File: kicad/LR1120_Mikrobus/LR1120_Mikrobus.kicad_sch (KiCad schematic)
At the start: 8 parts, among them IC1 BGA524N6E6327XTSA1, IC2 SKY13588-460LF, IC3 M24128-BFMH6TG, U1 LR1120, U4 LIS2DE12

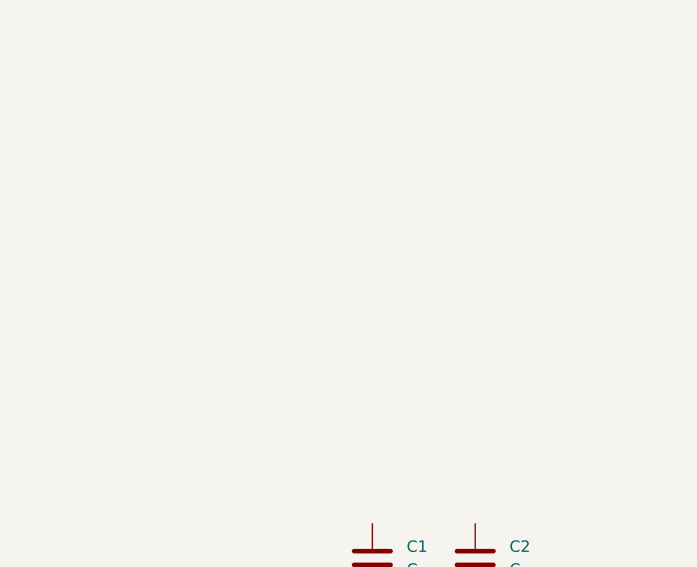
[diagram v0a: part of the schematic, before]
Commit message: Small corrections from last commit
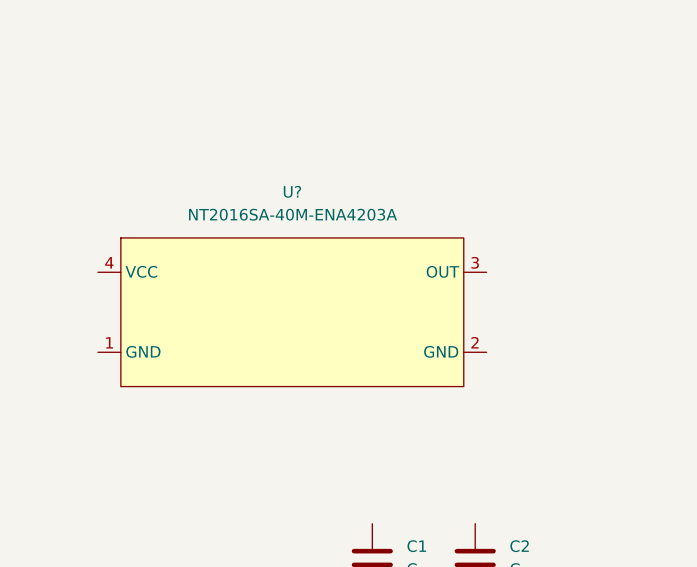
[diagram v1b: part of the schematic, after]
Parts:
- added U?: NT2016SA-40M-ENA4203A, symbol TCXO:NT2016SA-40M-ENA4203A
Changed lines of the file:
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@@
     (pin "9")
+  )
+  (symbol (lib_id "TCXO:NT2016SA-40M-ENA4203A") (at 57.15 66.04 0) (unit 1)
+    (in_bom yes) (on_board yes) (fields_autoplaced)
+    (property "Reference" "U?" (id 0) (at 58.42 53.34 0))
+    (property "Value" "NT2016SA-40M-ENA4203A" (id 1) (at 58.42 55.88 0))
+    (property "Footprint" "" (id 2) (at 57.15 66.04 0)
+      (effects (font (size 1.27 1.27)) hide)
+    )
+    (property "Datasheet" "" (id 3) (at 57.15 66.04 0)
+      (effects (font (size 1.27 1.27)) hide)
+    )
+    (pin "1")
+    (pin "2")
+    (pin "3")
+    (pin "4")
   )
   (symbol (lib_id "M24128-BFMH6TG:M24128-BFMH6TG") (at 233.68 85.09 0) (unit 1)
@@
       (reference "U4") (unit 1) (value "LIS2DE12") (footprint "Package_LGA:LGA-12_2x2mm_P0.5mm")
     )
+    (path "/ef4af352-5d7c-4ee8-a333-c7263e32c96e"
+      (reference "U?") (unit 1) (value "NT2016SA-40M-ENA4203A") (footprint "")
+    )
     (path "/30d9f59d-f72b-41c4-8214-d95fedfe532c"
